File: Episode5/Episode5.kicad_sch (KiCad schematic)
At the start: 1 part, among them U13 74LS07

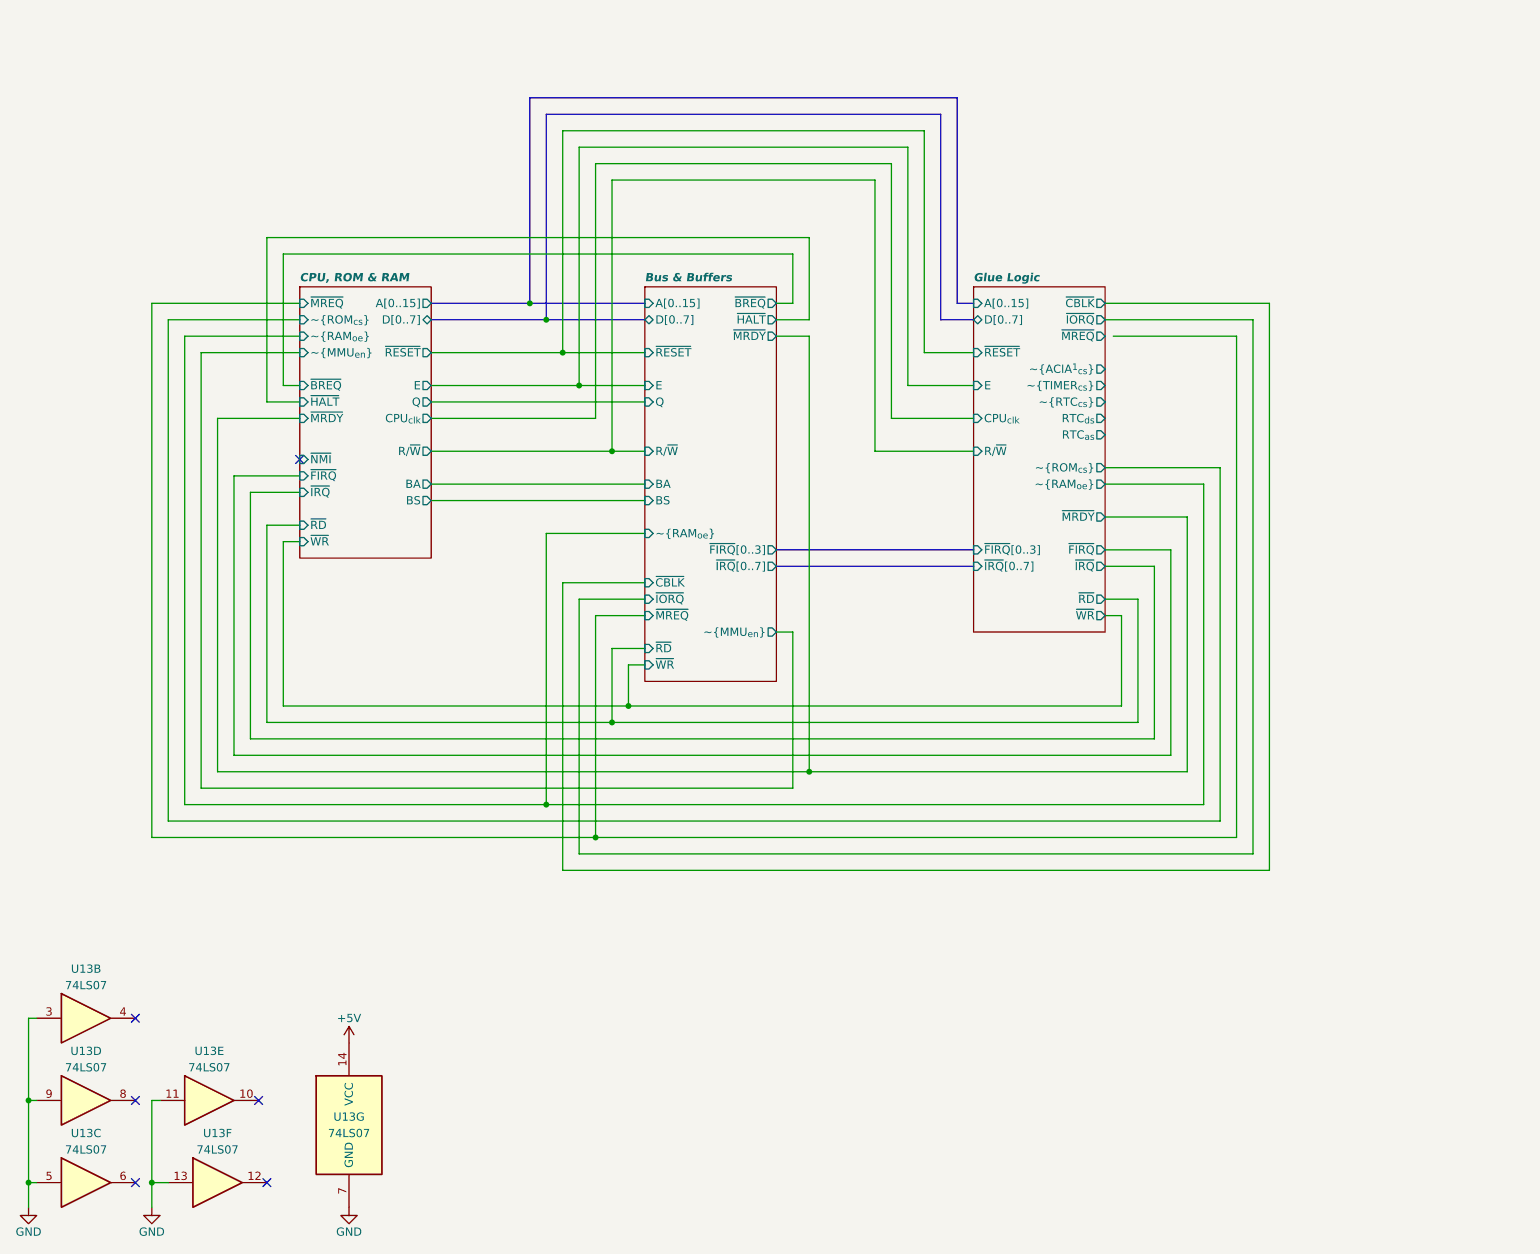
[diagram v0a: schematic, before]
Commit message: Finished the preliminary design of the CPU card
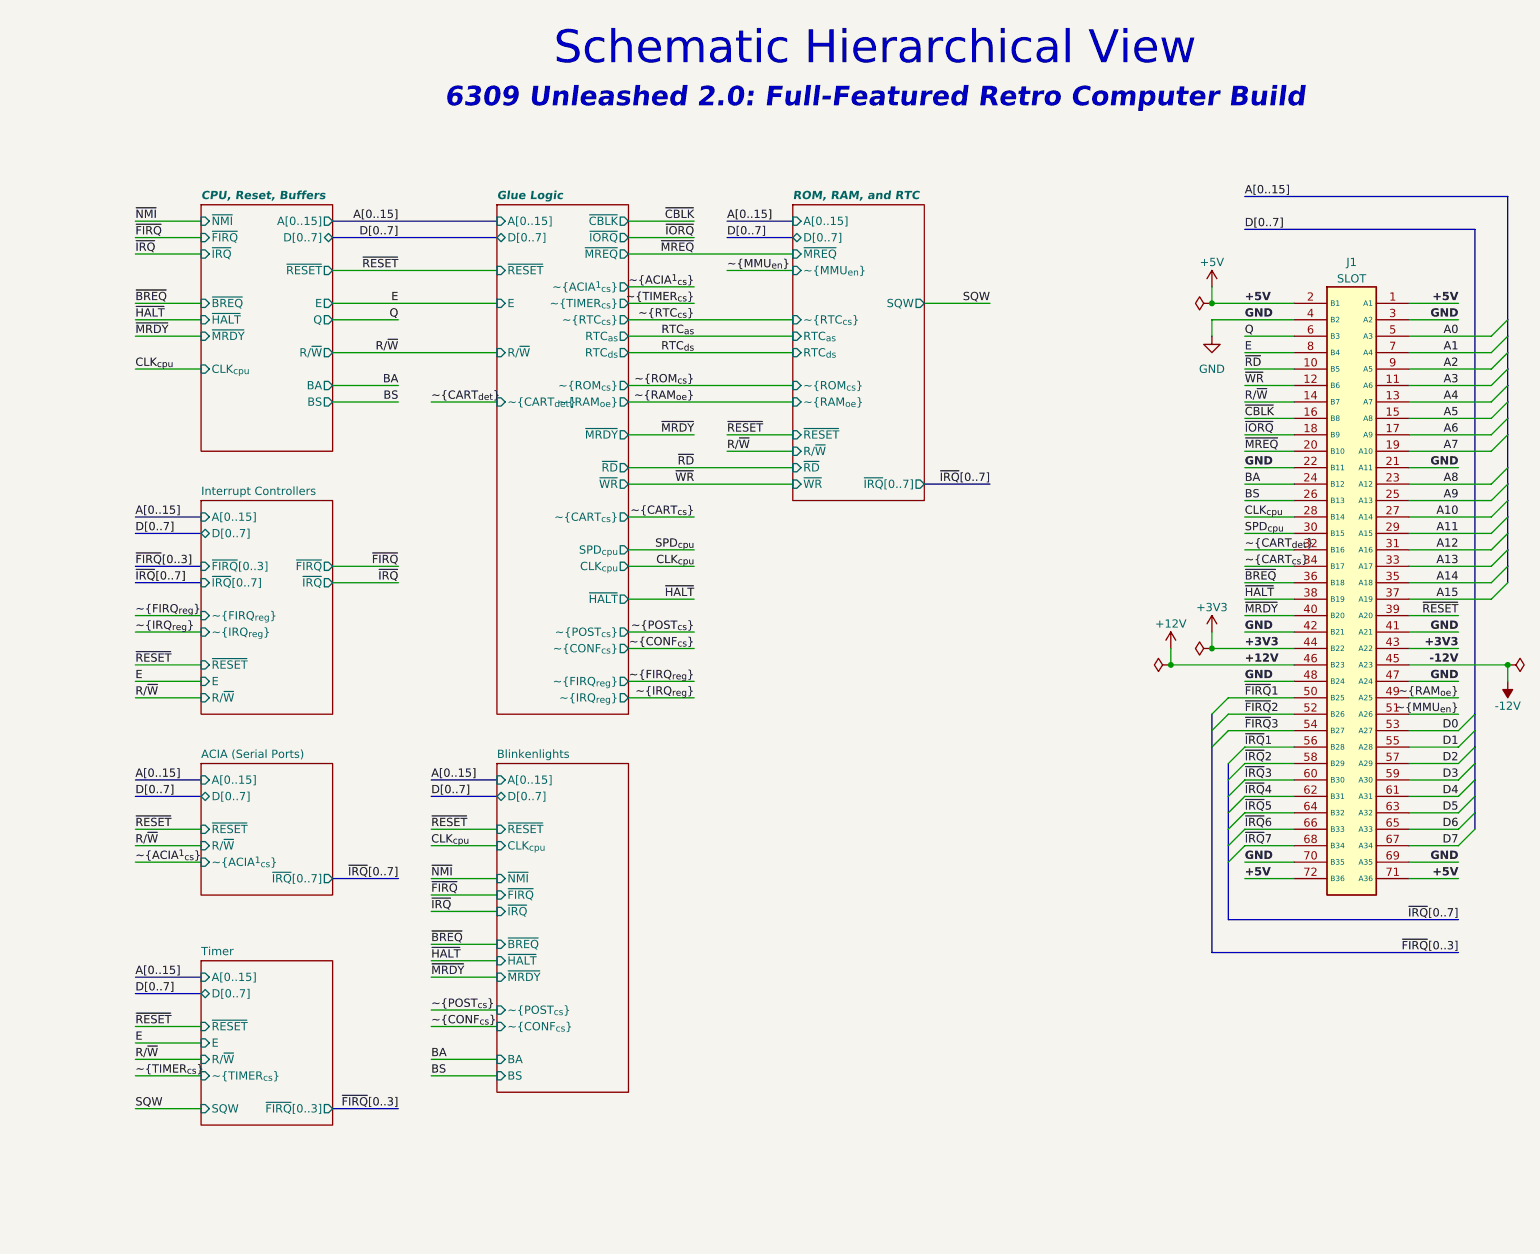
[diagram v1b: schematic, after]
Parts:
- removed U13: 74LS07, symbol 74xx:74LS07
- added J1: SLOT, MicroHobbyist:72-pin CE connector, symbol MicroHobbyist:72-pin Card Edge (ISA style)
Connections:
- net +5V: now also J1.1 (A1), J1.2 (B1), J1.71 (A36), J1.72 (B36)
- net GND: now also J1.21 (A11), J1.22 (B11), J1.3 (A2), J1.4 (B2), J1.41 (A21), J1.42 (B21), J1.47 (A24), J1.48 (B24), J1.69 (A35), J1.70 (B35)
- new net +12V: J1.46 (B23)
- new net +3V3: J1.43 (A22), J1.44 (B22)
- new net -12V: J1.45 (A23)
- new net A0: J1.5 (A3)
- new net A1: J1.7 (A4)
- new net A10: J1.27 (A14)
- new net A11: J1.29 (A15)
- new net A12: J1.31 (A16)
- new net A13: J1.33 (A17)
- new net A14: J1.35 (A18)
- new net A15: J1.37 (A19)
- new net A2: J1.9 (A5)
- new net A3: J1.11 (A6)
- new net A4: J1.13 (A7)
- new net A5: J1.15 (A8)
- new net A6: J1.17 (A9)
- new net A7: J1.19 (A10)
- new net A8: J1.23 (A12)
- new net A9: J1.25 (A13)
- new net BA: J1.24 (B12)
- new net BS: J1.26 (B13)
- new net CLK_{cpu}: J1.28 (B14)
- new net D0: J1.53 (A27)
- new net D1: J1.55 (A28)
- new net D2: J1.57 (A29)
- new net D3: J1.59 (A30)
- new net D4: J1.61 (A31)
- new net D5: J1.63 (A32)
- new net D6: J1.65 (A33)
- new net D7: J1.67 (A34)
- new net E: J1.8 (B4)
- new net Q: J1.6 (B3)
- new net R/~{W}: J1.14 (B7)
- new net SPD_{cpu}: J1.30 (B15)
- new net ~{BREQ}: J1.36 (B18)
- new net ~{CART_{cs}}: J1.34 (B17)
- new net ~{CART_{det}}: J1.32 (B16)
- new net ~{CBLK}: J1.16 (B8)
- new net ~{FIRQ}1: J1.50 (B25)
- new net ~{FIRQ}2: J1.52 (B26)
- new net ~{FIRQ}3: J1.54 (B27)
- new net ~{HALT}: J1.38 (B19)
- new net ~{IORQ}: J1.18 (B9)
- new net ~{IRQ}1: J1.56 (B28)
- new net ~{IRQ}2: J1.58 (B29)
- new net ~{IRQ}3: J1.60 (B30)
- new net ~{IRQ}4: J1.62 (B31)
- new net ~{IRQ}5: J1.64 (B32)
- new net ~{IRQ}6: J1.66 (B33)
- new net ~{IRQ}7: J1.68 (B34)
- new net ~{MMU_{en}}: J1.51 (A26)
- new net ~{MRDY}: J1.40 (B20)
- new net ~{MREQ}: J1.20 (B10)
- new net ~{RAM_{oe}}: J1.49 (A25)
- new net ~{RD}: J1.10 (B5)
- new net ~{RESET}: J1.39 (A20)
- new net ~{WR}: J1.12 (B6)
- no-connect marks 6 -> 0
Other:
- sheet Bus & Buffers renamed CPU, Reset, Buffers
- sheet CPU, ROM & RAM renamed ROM, RAM, and RTC
- added sheet ACIA (Serial Ports) (ACIA.kicad_sch)
- added sheet Blinkenlights (Blinkenlights.kicad_sch)
- added sheet Interrupt Controllers (Interrupts.kicad_sch)
- added sheet Timer (TIMER.kicad_sch)
- sheet CPU, Reset, Buffers ports: added CLK_{cpu}, ~{FIRQ}, ~{IRQ}, ~{NMI}; removed ~{CBLK}, ~{FIRQ}[0..3], ~{IORQ}, ~{IRQ}[0..7], ~{MMU_{en}}, ~{MREQ}, ~{RAM_{oe}}, ~{RD}, ~{WR}
- sheet Glue Logic ports: added CLK_{cpu}, SPD_{cpu}, ~{CART_{cs}}, ~{CART_{det}}, ~{CONF_{cs}}, ~{FIRQ_{reg}}, ~{HALT}, ~{IRQ_{reg}}, ~{POST_{cs}}; removed CPU_{clk}, ~{FIRQ}, ~{FIRQ}[0..3], ~{IRQ}, ~{IRQ}[0..7]
- sheet ROM, RAM, and RTC ports: added RTC_{as}, RTC_{ds}, SQW, ~{IRQ}[0..7], ~{RTC_{cs}}; removed BA, BS, CPU_{clk}, E, Q, ~{BREQ}, ~{FIRQ}, ~{HALT}, ~{IRQ}, ~{MRDY}, ~{NMI}
- note added: "6309 Unleashed 2.0: Full-Featured Retro Computer Build"
- note added: "Schematic Hierarchical View"
- company: Frédéric "MicroHobbyist" Segard -> MicroHobbyist
